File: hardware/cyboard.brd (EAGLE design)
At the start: 78.4 x 86.4 mm, 31 parts, among them CON1 CPCBUS, IC1 PIC16F84AP, IC2 74HCT21N, IC3 74HCT244N, IC4 GAL20V8B, IC5 DS12887A

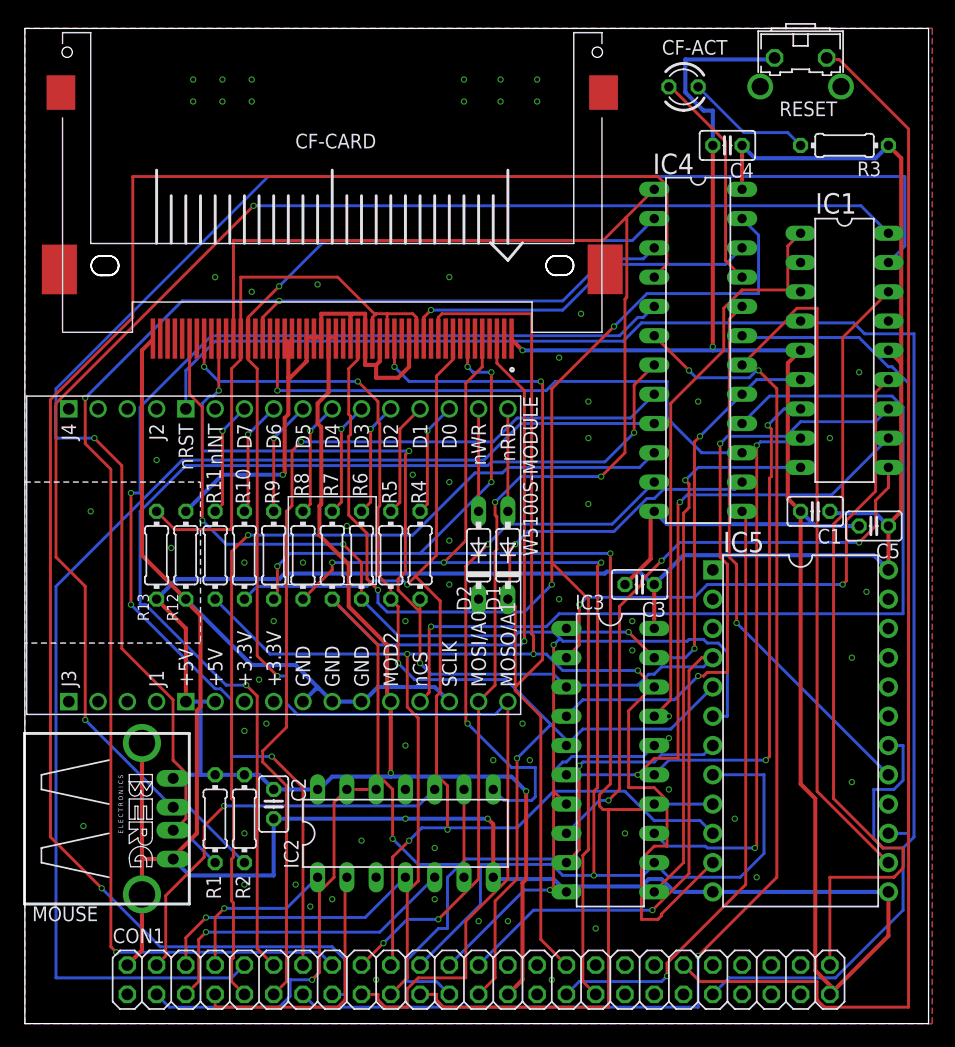
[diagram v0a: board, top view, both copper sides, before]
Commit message: Add files via upload
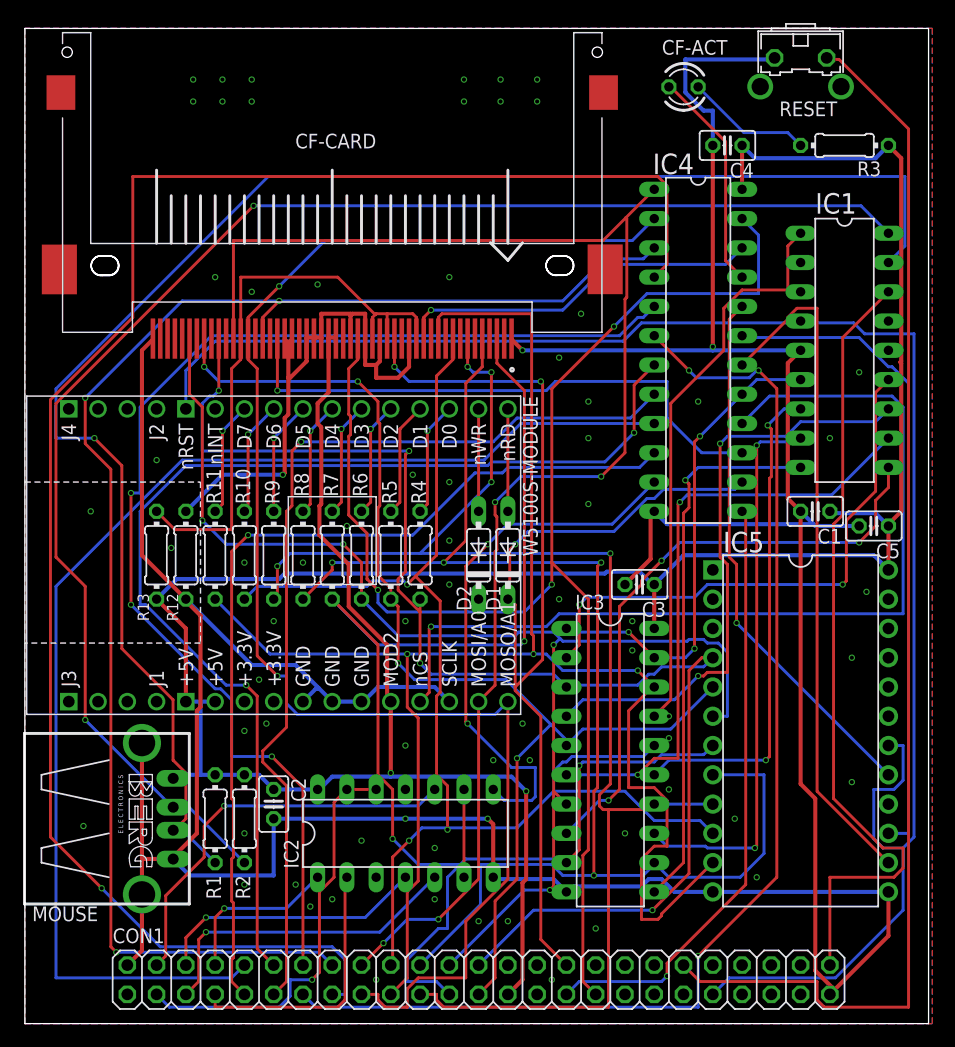
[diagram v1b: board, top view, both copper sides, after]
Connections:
- net /A3 renamed CFA3
- net /MOUSEINT renamed /PINT
- net ADDR1015 renamed A1X
